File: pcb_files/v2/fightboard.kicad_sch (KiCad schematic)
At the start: 34 parts, among them J1 SW_Push, K1 SW_Push, M1 XIAO-RP2040, P1 SW_Push, U1 SW_Push

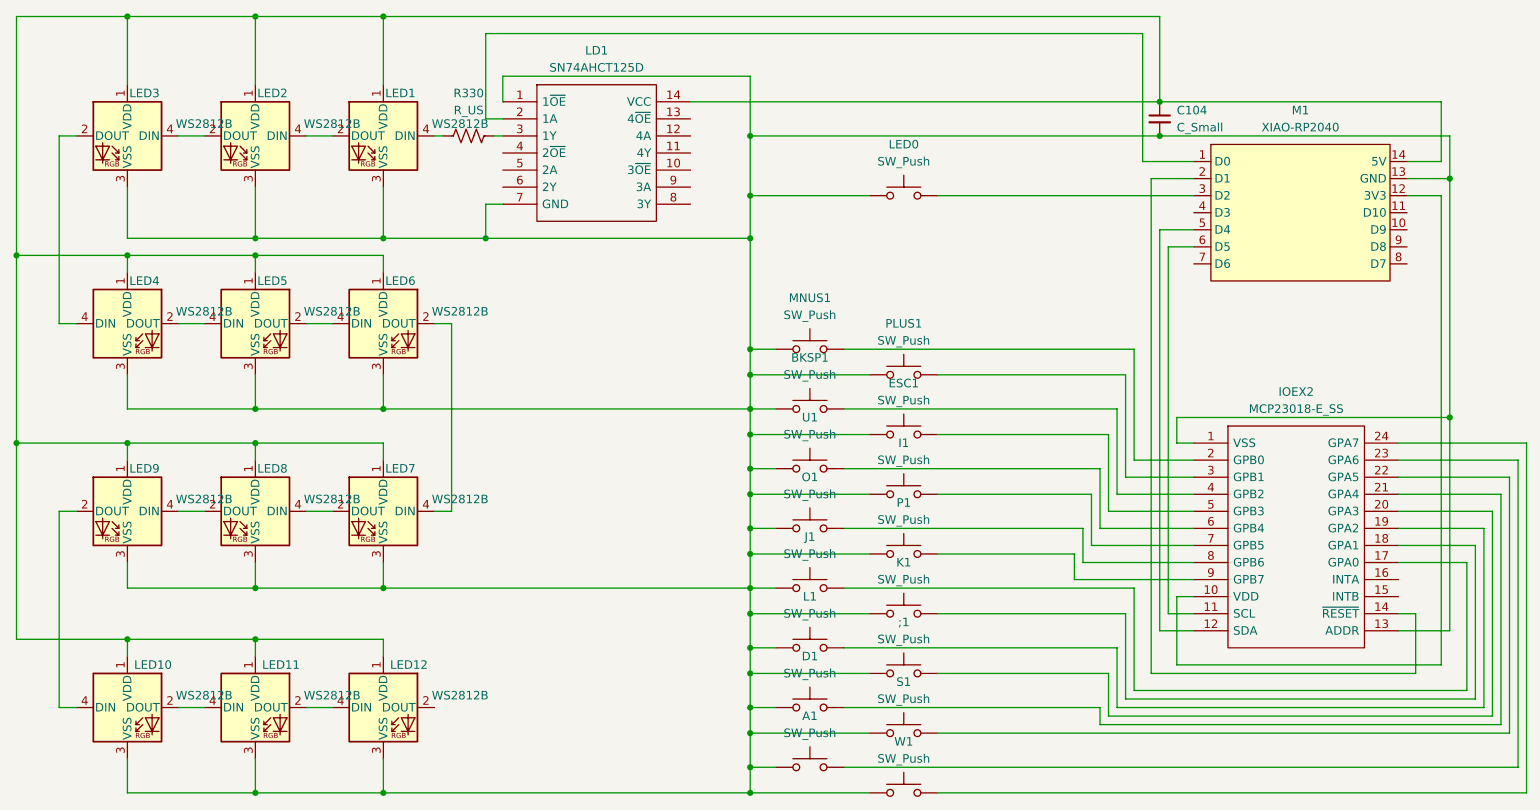
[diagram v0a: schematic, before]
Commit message: update v2 pcb
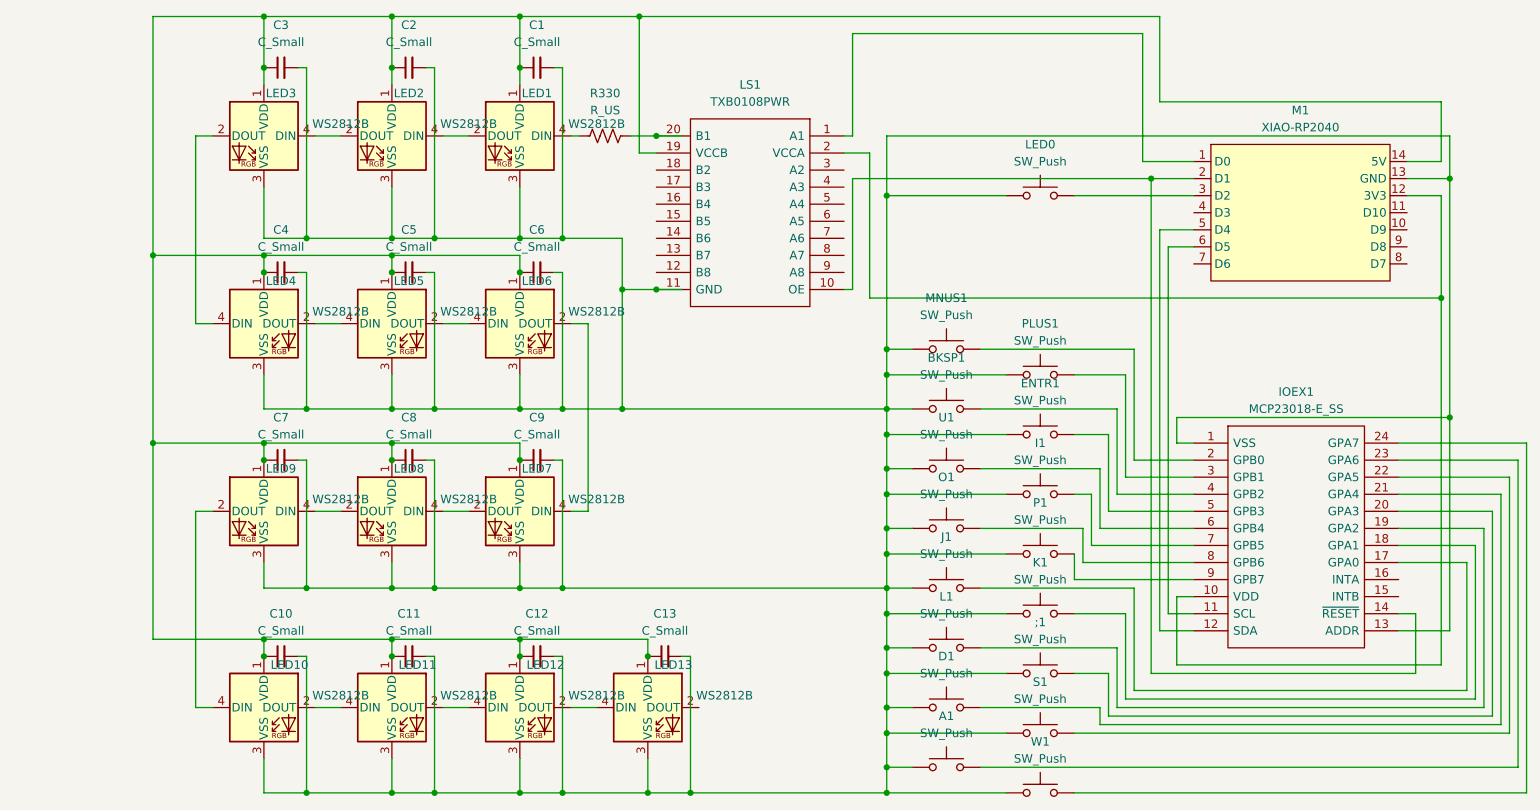
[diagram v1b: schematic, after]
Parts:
- removed C104: C_Small, Resistor_SMD:R_2010_5025Metric_Pad1.40x2.65mm_HandSolder, symbol Device:C_Small
- removed LD1: SN74AHCT125D, SOIC127P600X175-14N, symbol SN74HCT125D:SN74AHCT125D
- added C1, C10, C11, C12, C13, C2, C3, C4, C5, C6, C7, C8, C9: C_Small, Resistor_SMD:R_2010_5025Metric_Pad1.40x2.65mm_HandSolder, symbol Device:C_Small
- added LED13: WS2812B, kb_lib:Reverse Mount SK6812MINI-E, symbol LED:WS2812B
- added LS1: TXB0108PWR, SOP65P640X120-20N, symbol TXB0108PWR:TXB0108PWR
- renumbered ESC1 to ENTR1, IOEX2 to IOEX1
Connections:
- net at ;1.1, A1.1, BKSP1.1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: now also C1.2, C10.2, C11.2, C12.2, C13.2, C2.2, C3.2, C4.2, C5.2, C6.2, C7.2, C8.2, C9.2, LED13.3 (VSS), LS1.11 (GND)
- net at LED1.1 (VDD), LED10.1 (VDD), LED11.1 (VDD)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: now also C1.1, C10.1, C11.1, C12.1, C13.1, C2.1, C3.1, C4.1, C5.1, C6.1, C7.1, C8.1, C9.1, LED13.1 (VDD), LS1.19 (VCCB)
- net at M1.1 (D0): now also LS1.1 (A1)
- net at R330.2: now also LS1.20 (B1)
- net at IOEX1.10 (VDD), M1.12 (3V3): now also LS1.2 (VCCA)
- net at IOEX1.14 (~{RESET}), M1.2 (D1): now also LS1.10 (OE)
- net at LED12.2 (DOUT): now also LED13.4 (DIN)
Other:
- moved on the sheet: ;1, A1, BKSP1, D1, ENTR1, I1, J1, K1, L1, LED0, LED1, LED10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
